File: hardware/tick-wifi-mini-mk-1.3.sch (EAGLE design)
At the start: 12 parts, among them IC1 HT16K33, U1 Adafruit Feather HUZZAH ESP82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

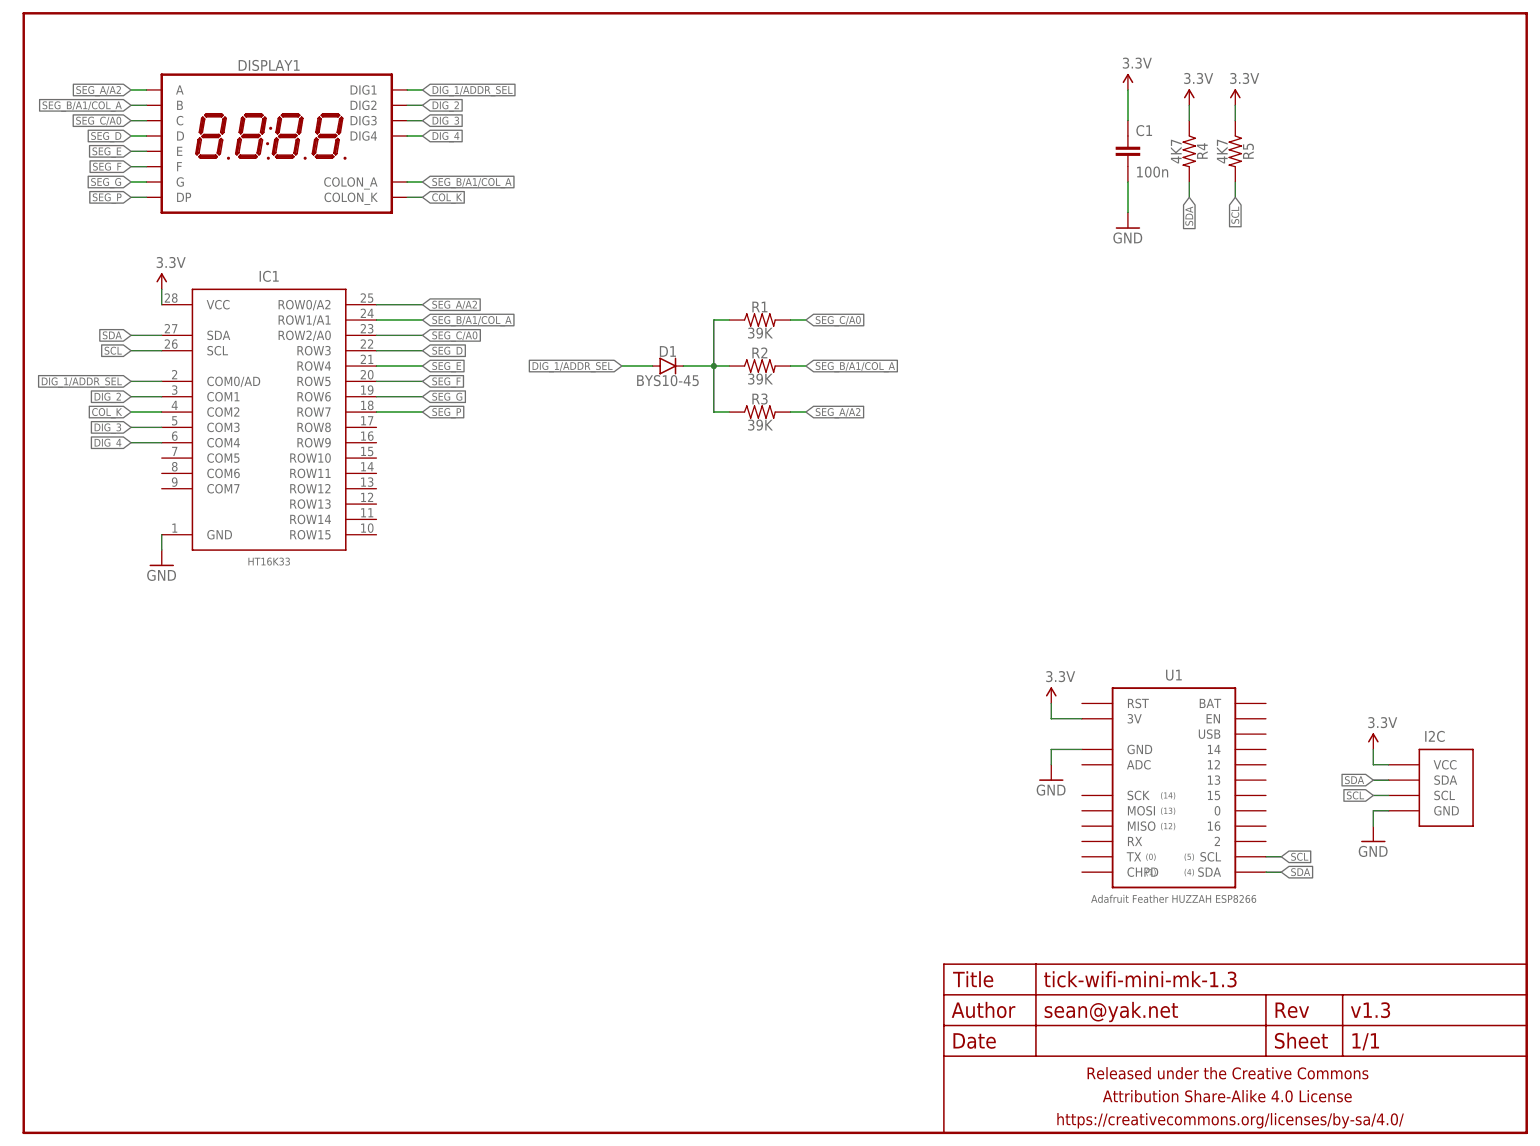
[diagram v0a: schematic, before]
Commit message: yet another attempt at a ht16k33 driver
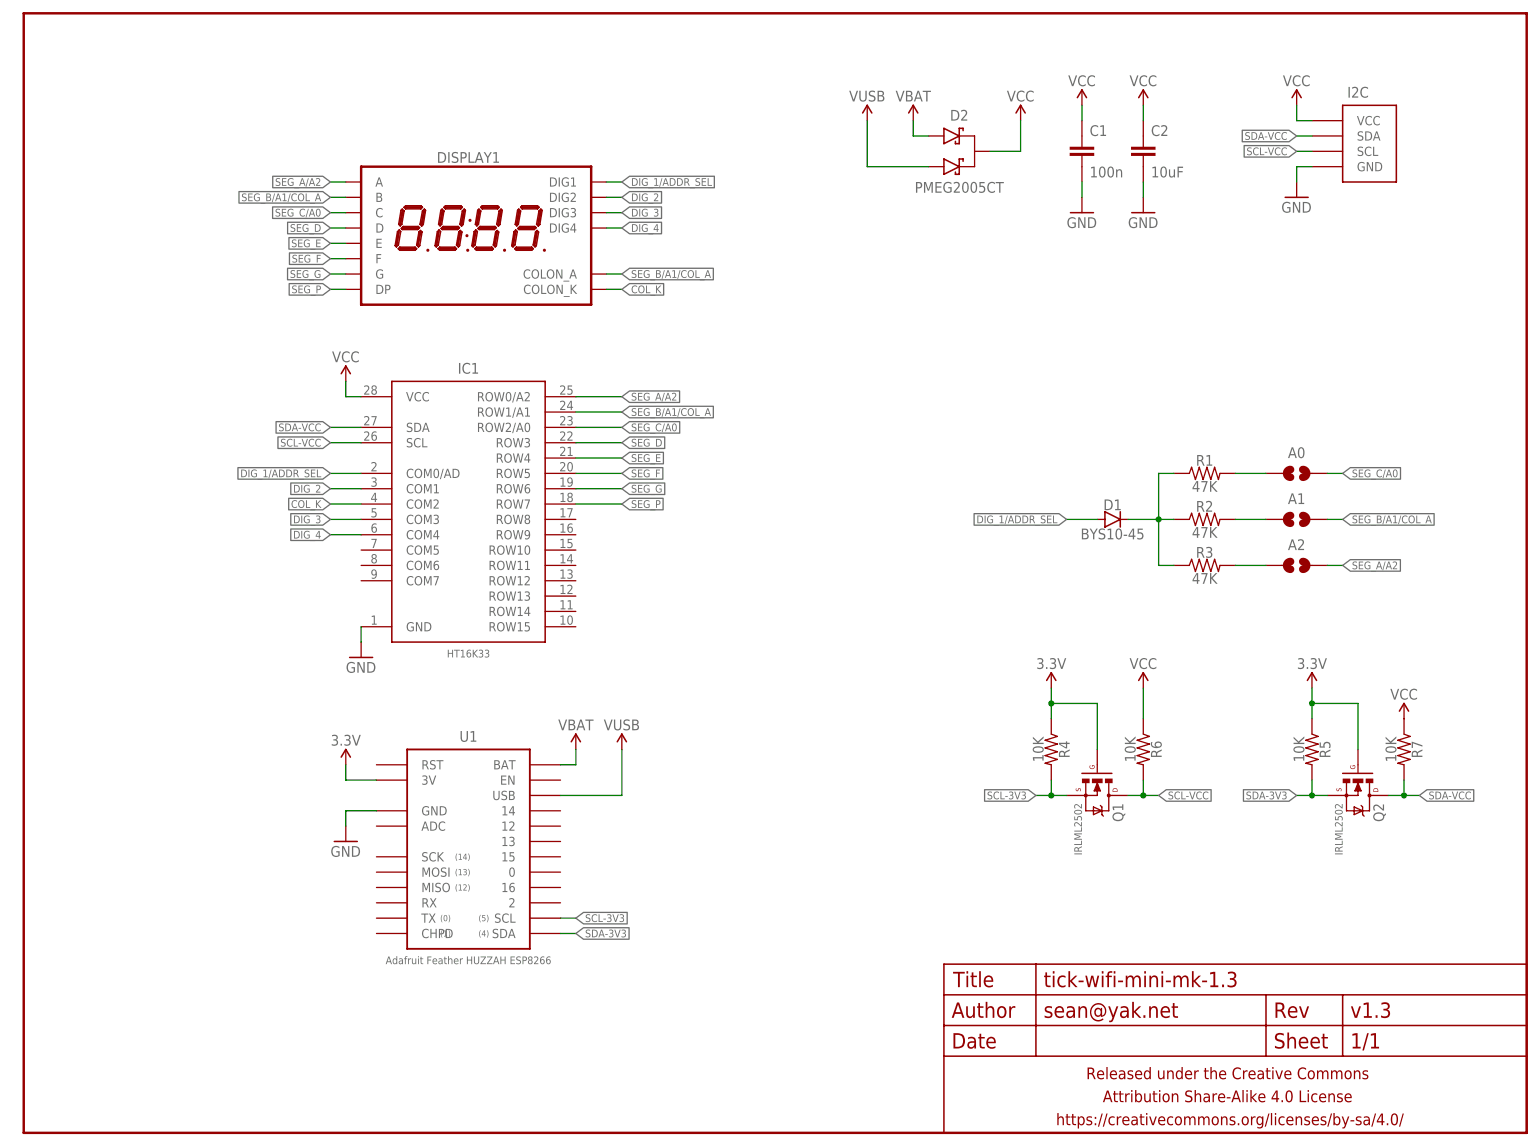
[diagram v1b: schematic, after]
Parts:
- added A0, A1, A2: JUMPER-PAD-2-NOYES_SILK, a_parts:JUMPER-PAD-2-NOYES_SILK
- added C2: 10uF, a_parts:CAPACITOR-CERAMICC0805-TIGHTER
- added D2: PMEG2005CT, a_parts:DIODE-SCHOTTKY-DUALPMEG2005CT
- added Q1, Q2: IRLML2502, a_parts:MOSFET-NCHANNELIRLML2502
- added R6, R7: 10K, a_parts:RESISTORR0603-TIGHTER
- C1: device a_parts:CAPACITOR-CERAMICC0805 -> a_parts:CAPACITOR-CERAMICC0603-TIGHTER
- D1: device a_parts:DIODESOD123 -> a_parts:DIODESOD
- I2C: value M04-I2CJST-4-PH-VERT-CENTERED-I2C -> M04-I2CPTH-2MM-CENTERED; device a_parts:M04-I2CJST-4-PH-VERT-CENTERED-I2C -> a_parts:M04-I2CPTH-2MM-CENTERED
- R1, R2, R3: value 39K -> 47K; device a_parts:RESISTORR0805 -> a_parts:RESISTORR0603-TIGHTER
- R4, R5: value 4K7 -> 10K; device a_parts:RESISTORR0805 -> a_parts:RESISTORR0603-TIGHTER
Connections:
- removed net SCL: I2C.SCL, IC1.SCL, R5.2, U1.SCL
- removed net SDA: I2C.SDA, IC1.SDA, R4.2, U1.SDA
- new net N$2: A0.1, R1.2
- new net N$3: A1.1, R2.2
- new net N$4: A2.1, R3.2
- new net SCL-3V3: Q1.S, R4.2, U1.SCL
- new net SCL-VCC: I2C.SCL, IC1.SCL, Q1.D, R6.2
- new net SDA-3V3: Q2.S, R5.2, U1.SDA
- new net SDA-VCC: I2C.SDA, IC1.SDA, Q2.D, R7.2
- new net VBAT: D2.A1, U1.BAT
- new net VCC: C1.1, C2.1, D2.K, I2C.VCC, IC1.VCC, R6.1, R7.1
- new net VUSB: D2.A2, U1.USB
- net 3.3V: now also Q1.G, Q2.G; no longer C1.1, I2C.VCC, IC1.VCC
- net GND: now also C2.2
- net SEG_A/A2: now also A2.2; no longer R3.2
- net SEG_B/A1/COL_A: now also A1.2; no longer R2.2
- net SEG_C/A0: now also A0.2; no longer R1.2
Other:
- moved on the sheet: C1, D1, DISPLAY1, I2C, IC1, R1, R2, R3, R4, R5, U1
